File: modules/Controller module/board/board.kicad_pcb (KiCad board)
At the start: 2 copper layers, 50 x 30 mm, 66 parts, among them IC1 DW01A, J1 Conn_01x05_Female, J2 Conn_01x04_Female, J3 Conn_01x04_Female, J4 Conn_01x02, J5 Conn_01x06_Female, J6 Conn_01x02_Female, J7 Conn_01x08_Female, P1 USB_C_Plug_USB2.0, Q1 AO3400A, Q2 AO3400A, Q3 AO3401A, Q4 FS8205A, SW1 SW_Push, SW2 SW_Push, SW3 SW_SPST, U1 ME6211, U2 ESP32-WROOM-32D, U3 TP4056, U4 MPU-6050

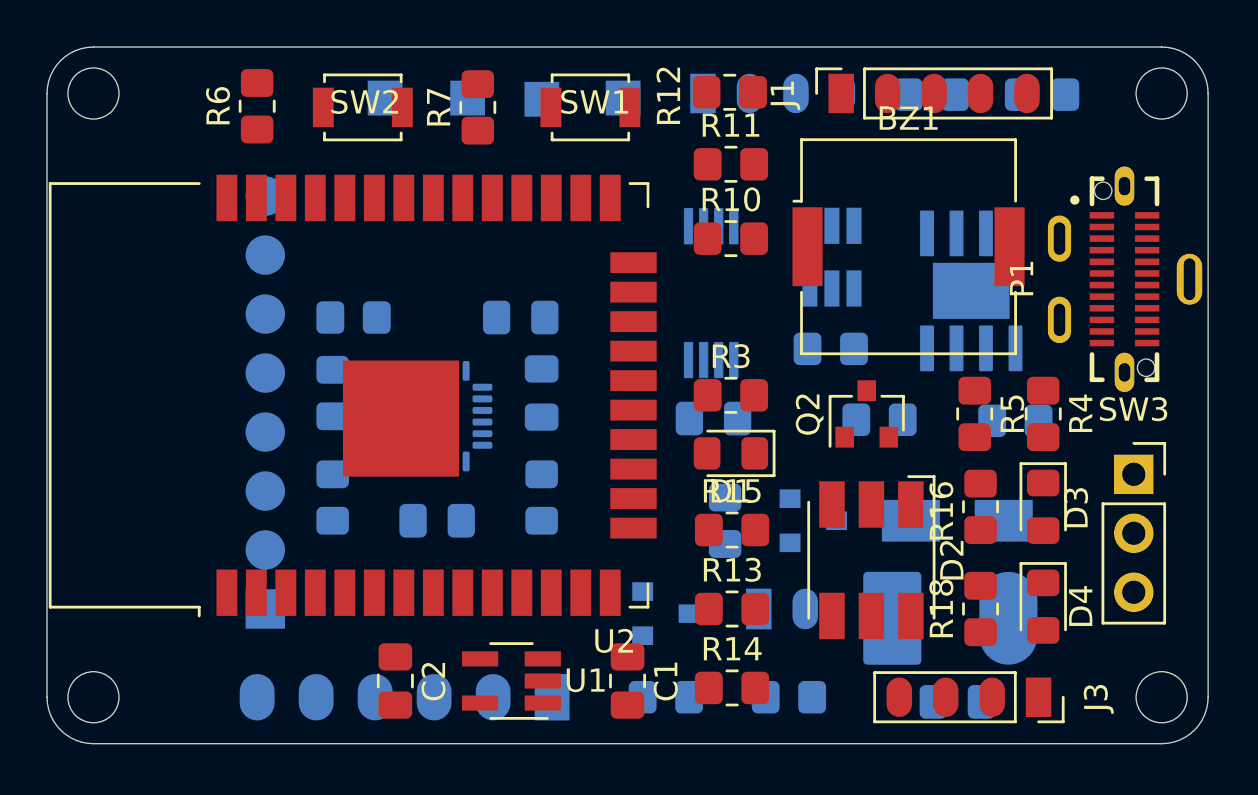
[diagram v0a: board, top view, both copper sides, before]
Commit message: Controller module: PCB complete
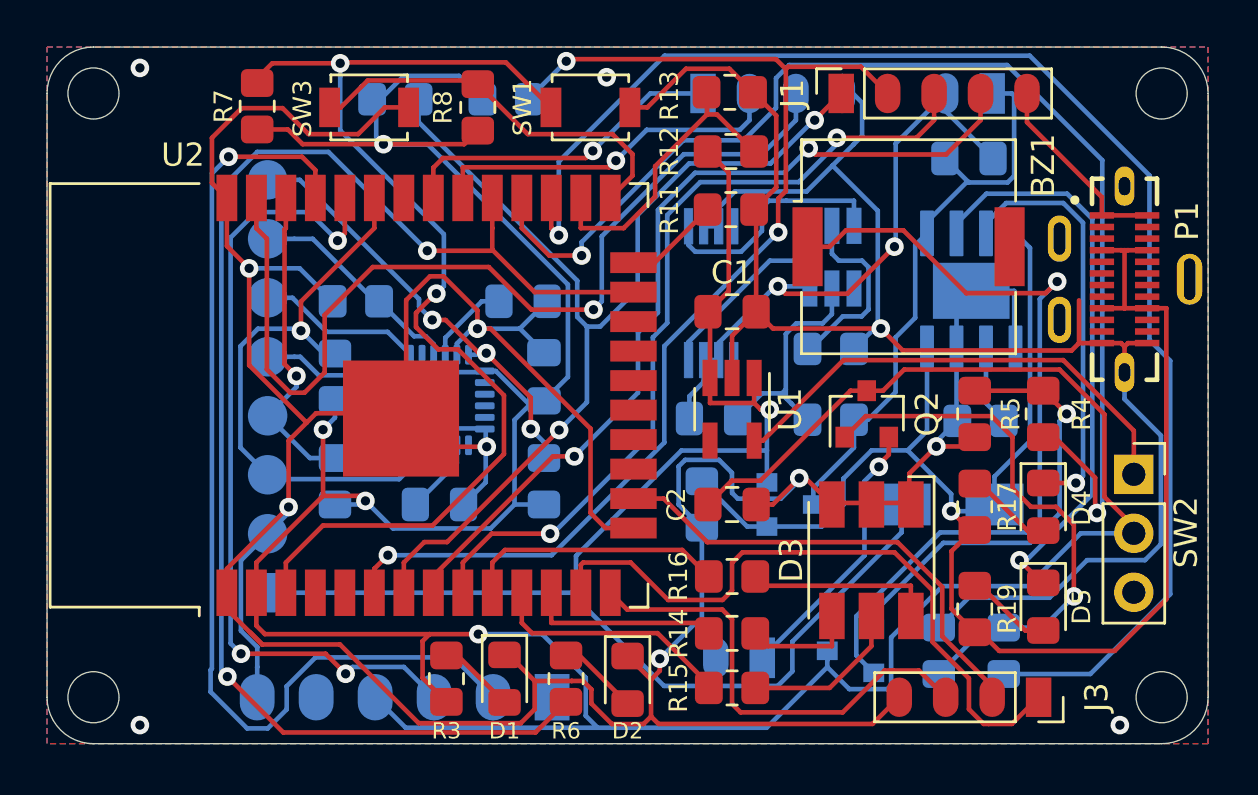
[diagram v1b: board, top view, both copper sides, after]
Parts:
- removed TP1, TP2, TP3, TP4: TestPoint, TestPoint:TestPoint_Pad_1.5x1.5mm
- added D2: LED, LED_SMD:LED_0805_2012Metric_Pad1.15x1.40mm_HandSolder, F.Cu at (130.0, 113.2)
- added R6: 10k, Resistor_SMD:R_0805_2012Metric_Pad1.20x1.40mm_HandSolder, F.Cu at (127.3, 113.2)
- J6: footprint Board:SolderWire-SMD-BATT -> Board:SolderWire_1x02_P2.00mm
- U2: footprint RF_Module:ESP32-WROOM-32 -> Board:ESP32-WROOM-32
- moved C4 23.4 mm to (144.7, 90.8)
- moved R1 23.1 mm to (120.0, 88.2)
- moved R2 23.1 mm to (124.8, 88.2)
- moved J6 23.0 mm to (145.7, 88.0), turned to 90 degrees
- moved R3 17.3 mm to (122.2, 113.2), turned to 90 degrees
- moved C1 16.5 mm to (134.5, 97.4), turned to 0 degrees
- moved C2 16.4 mm to (134.5, 105.7), turned to 0 degrees
- moved U1 15.1 mm to (134.5, 101.6), turned to 270 degrees
- moved D1 13.8 mm to (124.7, 113.2), turned to 270 degrees
- moved R10 11.9 mm to (143.4, 112.0), turned to 90 degrees
- moved R9 9.46 mm to (146.2, 112.0), turned to 270 degrees
- moved Q1 8.11 mm to (139.6, 112.0), turned to 180 degrees
- moved J4 2.11 mm to (135.8, 112.3), turned to 90 degrees
- moved R20 2.10 mm to (138.8, 102.0)
- moved R16 2.00 mm to (134.5, 108.8)
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- renumbered D2 to D3, D3 to D4, D4 to D5, D5 to D6, R9 to R10, R10 to R11, R11 to R12, R12 to R13, R13 to R14, R14 to R15, R15 to R16, R16 to R17, R17 to R18, R18 to R19, R19 to R20, R20 to R21, R21 to R22, R22 to R23, R23 to R24, R24 to R25, R25 to R26, R6 to R7, R7 to R8, R8 to R9, SW3 to SW2, SW2 to SW3
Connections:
- J7 pad 1: +3V3 -> VCC
- U2 pad 23: (no net) -> /IO15
- U2 pad 29: (no net) -> /IO15
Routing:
- net GND: track 0.00 -> 267.3 mm, vias 0 -> 12
- net +3V3: track 0.00 -> 153.9 mm, vias 0 -> 4
- net +5V: track 0.00 -> 70.2 mm, vias 0 -> 1
- net VCC: track 0.00 -> 64.0 mm, vias 0 -> 1
- net /IO16: track 0.00 -> 61.4 mm, vias 0 -> 1
- net /IO15: track 0.00 -> 60.4 mm, vias 0 -> 2
- net /BUZZER: track 0.00 -> 52.8 mm, vias 0 -> 2
- net /BTN2: track 0.00 -> 50.9 mm, vias 0 -> 3
- net /EN: track 0.00 -> 47.1 mm, vias 0 -> 2
- net /BTN1: track 0.00 -> 45.1 mm, vias 0 -> 2
- net /TX: track 0.00 -> 43.9 mm, vias 0 -> 1
- net /BTN-C: track 0.00 -> 41.4 mm, vias 0 -> 1
- net /BTN4: track 0.00 -> 37.9 mm, vias 0 -> 2
- net /BTN3: track 0.00 -> 35.9 mm, vias 0 -> 2
- net Net-(BZ1-Pad1): track 0.00 -> 35.3 mm, vias 0 -> 1
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- added copper zone on B.Cu, net GND
- added copper zone on F.Cu, net GND
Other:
- net class Default: trace_width 0.25 -> 0.2
